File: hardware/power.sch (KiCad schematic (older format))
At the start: 18 parts, among them U3 AMS1117-3.3

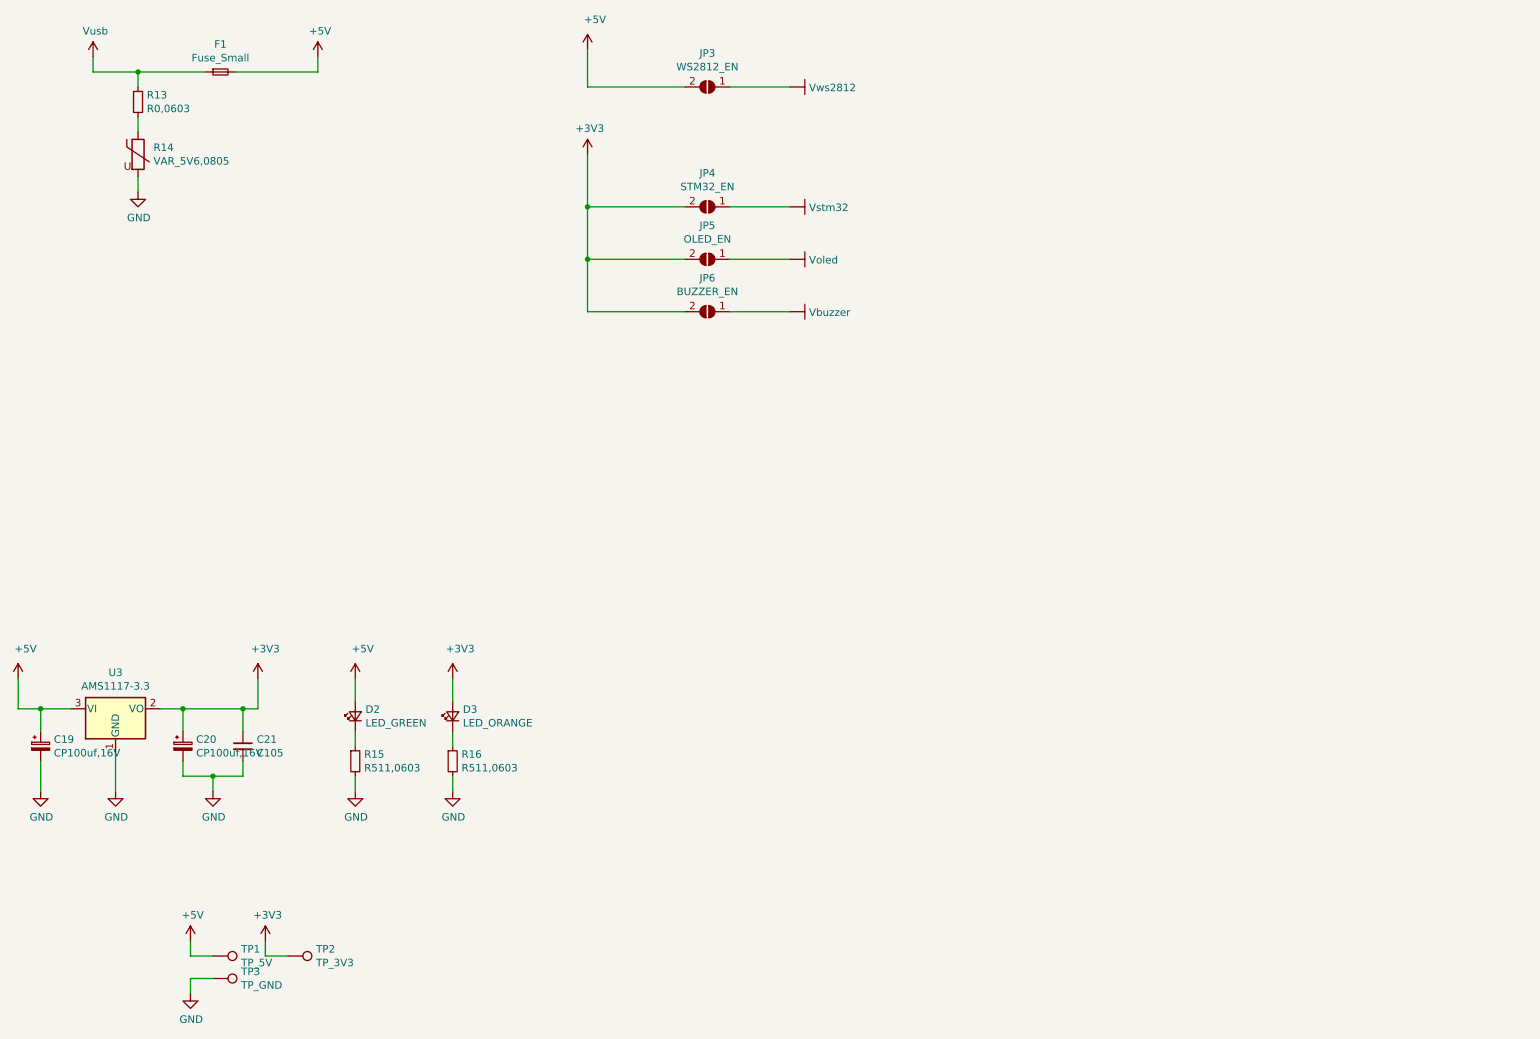
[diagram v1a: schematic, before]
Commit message: update,
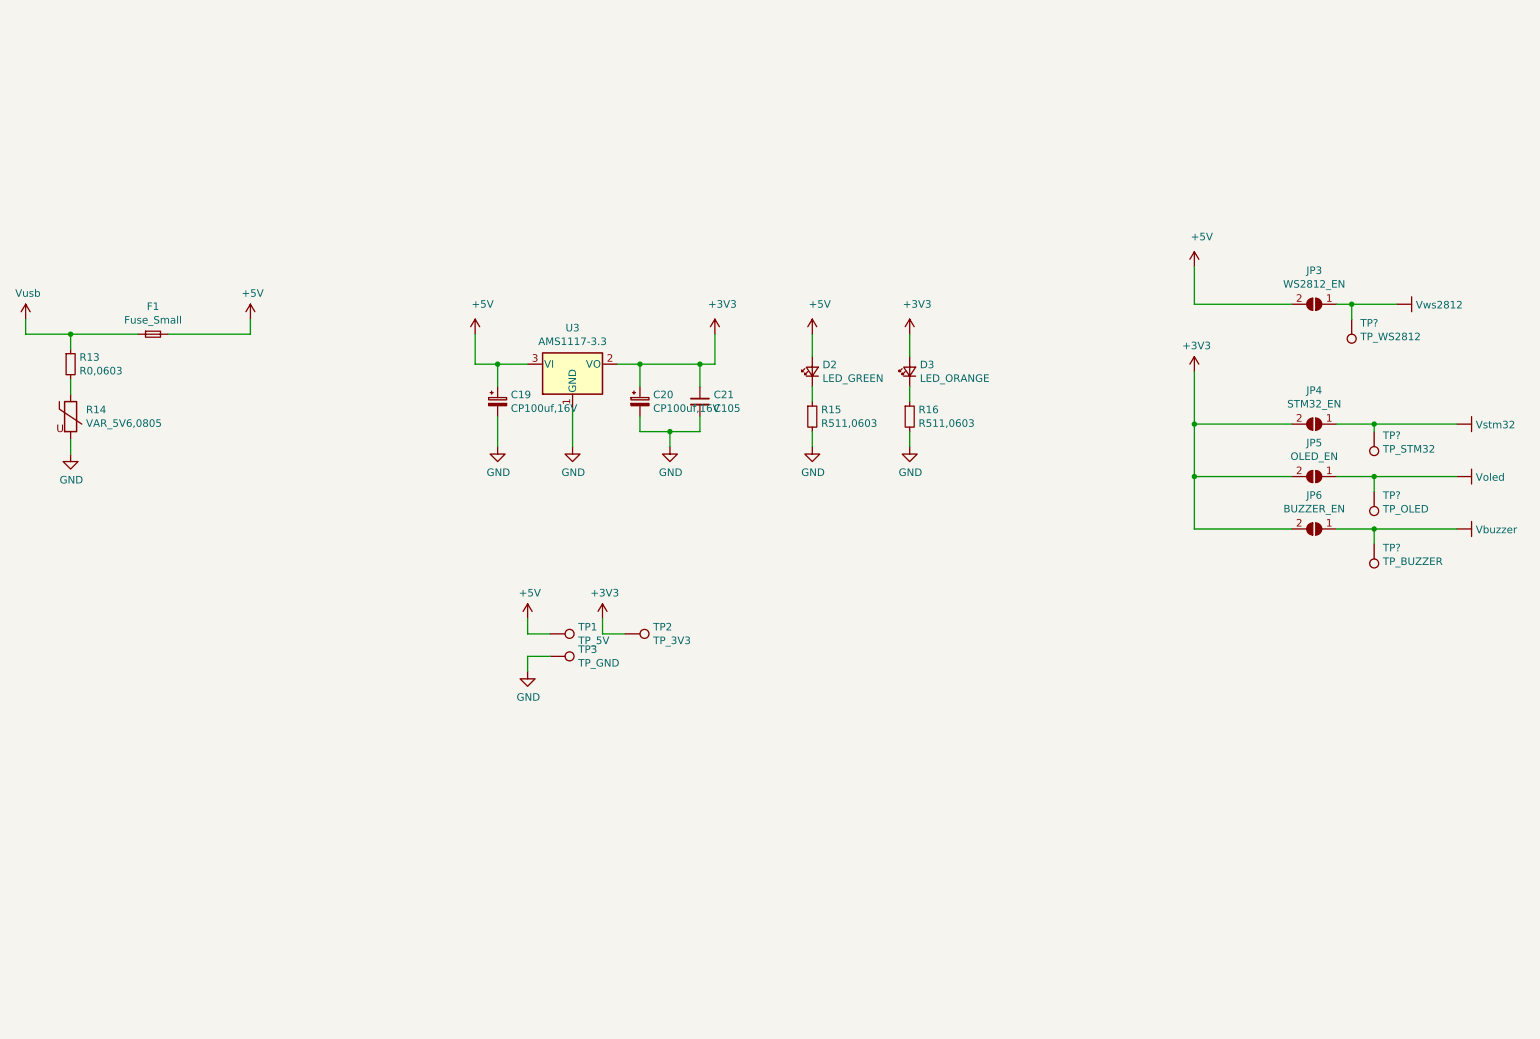
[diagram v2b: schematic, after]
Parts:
- added TP?: TP_BUZZER, TestPoint:TestPoint_THTPad_D2.0mm_Drill1.0mm, symbol my_testpoint:TestPoint_2mm
- added TP?: TP_OLED, TestPoint:TestPoint_THTPad_D2.0mm_Drill1.0mm, symbol my_testpoint:TestPoint_2mm
- added TP?: TP_STM32, TestPoint:TestPoint_THTPad_D2.0mm_Drill1.0mm, symbol my_testpoint:TestPoint_2mm
- added TP?: TP_WS2812, TestPoint:TestPoint_THTPad_D2.0mm_Drill1.0mm, symbol my_testpoint:TestPoint_2mm
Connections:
- net Vbuzzer: now also TP?.1
- net Voled: now also TP?.1
- net Vstm32: now also TP?.1
- net Vws2812: now also TP?.1
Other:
- moved on the sheet: C19, C20, C21, D2, D3, F1, JP3, JP4, JP5, JP6, R13, R14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
